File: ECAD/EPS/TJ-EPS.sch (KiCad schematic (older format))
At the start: 41 parts, among them J1 SWD, J2 BOOT, Q1 2N7002, Q2 IRF7425, U1 CD74HC4067SM, U2 MAX6369, U3 CD74HC4067SM, U4 STM32F103C8Tx, U60 CD74HC4067SM, Y1 8MHz

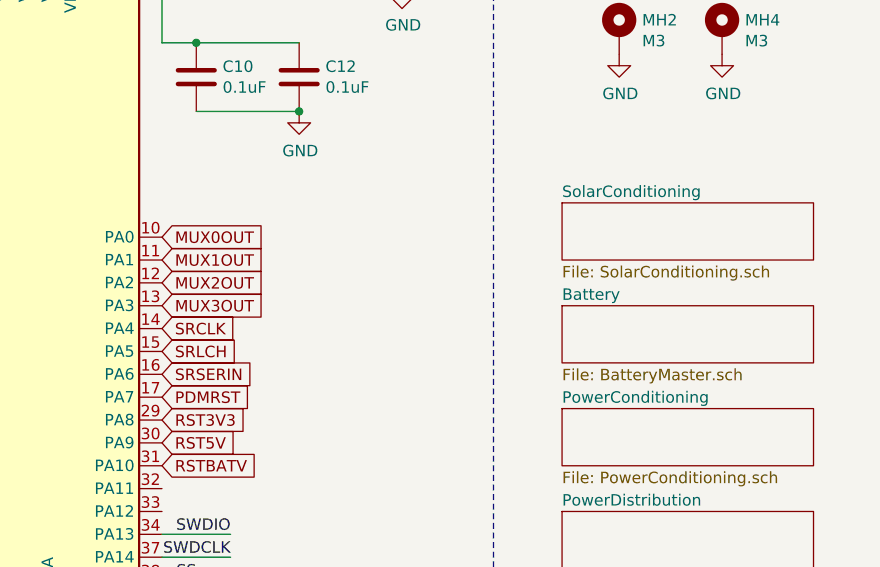
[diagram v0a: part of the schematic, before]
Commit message: Split up into 3 projects for separate boards
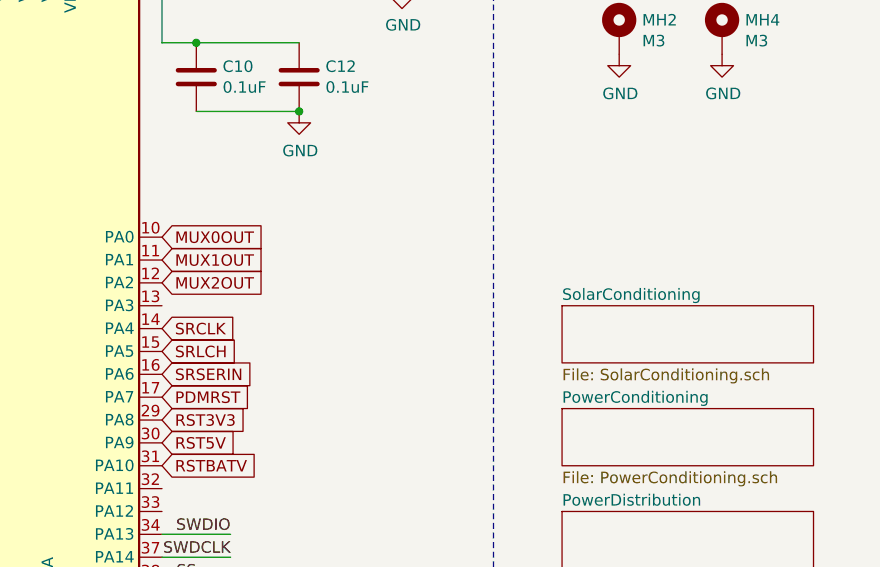
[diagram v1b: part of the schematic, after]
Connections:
- net MUX3OUT: no longer names the net of U4.13 (PA3)
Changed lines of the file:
@@
 $Descr USLegal 14000 8500
 encoding utf-8
-Sheet 1 37
+Sheet 1 32
 Title "TJ Custom EPS"
 Date ""
@@
 $Sheet
 S 10400 2550 1100 250
-U 61BD4B7D
-F0 "Battery" 50
-F1 "BatteryMaster.sch" 50
-$EndSheet
-$Sheet
-S 10400 2100 1100 250
 U 61BEC565
 F0 "SolarConditioning" 50
@@
 Text GLabel 8650 2450 2    50   Input ~ 0
 MUX2OUT
-Text GLabel 8650 2550 2    50   Input ~ 0
-MUX3OUT
 Text GLabel 8650 3250 2    50   Input ~ 0
 RSTBATV
